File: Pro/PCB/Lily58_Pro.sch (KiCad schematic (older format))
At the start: 83 parts, among them J1 LED, J2 4PIN, J3 OLED, P1 i2c_pin, P2 i2c_pin, SW1 SW_PUSH, SW10 SW_PUSH, SW11 SW_PUSH, SW12 SW_PUSH, SW13 SW_PUSH, SW14 SW_PUSH, SW15 SW_PUSH, SW16 SW_PUSH, SW17 SW_PUSH, SW18 SW_PUSH, SW19 SW_PUSH, SW2 SW_PUSH, SW20 SW_PUSH, SW21 SW_PUSH, SW22 SW_PUSH, SW23 SW_PUSH, SW24 SW_PUSH, SW25 SW_PUSH, SW26 SW_PUSH, SW27 SW_PUSH, SW28 SW_PUSH, SW29 SW_PUSH, SW3 SW_PUSH, SW4 SW_PUSH, SW5 SW_PUSH, SW6 SW_PUSH, SW7 SW_PUSH, SW8 SW_PUSH, SW9 SW_PUSH, U1 ProMicro

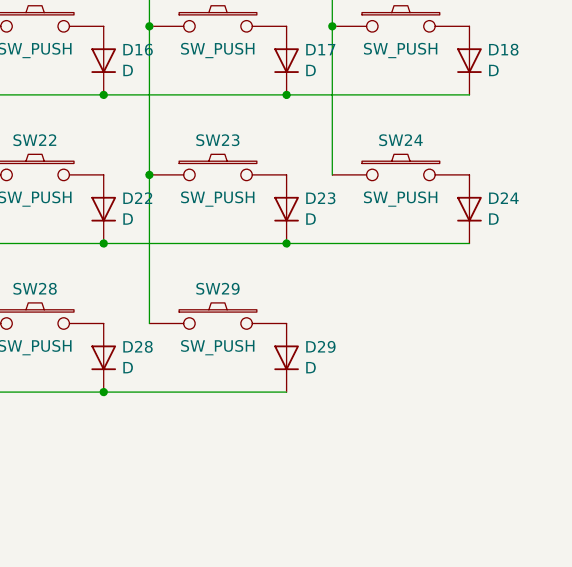
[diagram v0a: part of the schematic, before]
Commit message: Add another switch.
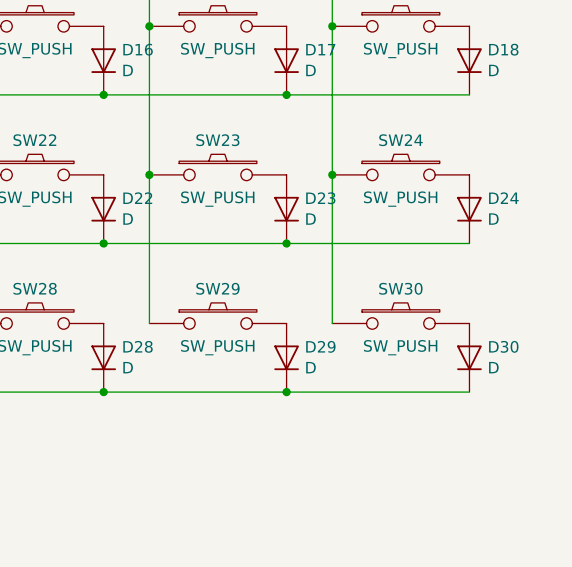
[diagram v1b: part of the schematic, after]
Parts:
- added D30: D, Lily58-footprint:Diode_SOD123, symbol Lily58_Pro-rescue:D-Lily58-cache
- added SW30: SW_PUSH, Lily58-footprint:CherryMX_KailhLowProfile_Hotswap, symbol Lily58_Pro-rescue:SW_PUSH-Lily58-cache
- SW1, SW10, SW11, SW12, SW13, SW14, SW15, SW16, SW17, SW18, SW19, SW2, SW20, SW21, SW22, SW23, SW24, SW25, SW27, SW28, SW29, SW3, SW4, SW5, SW6, SW7, SW8, SW9: footprint Lily58-footprint:CherryMX_KailhLowProfile_Hotswap_edge_fixed -> Lily58-footprint:CherryMX_KailhLowProfile_Hotswap
- SW26: footprint Lily58-footprint:CherryMX_KailhLowProfile_Hotswap_edge_fixed -> Lily58-footprint:CherryMX_KailhLowProfile_Hotswap_1.5
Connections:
- net col0: now also SW30.1
- net row4: now also D30.1 (K)
- new net: D30.2 (A), SW30.2
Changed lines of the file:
@@
 F 0 "SW25" H 5800 5000 50  0000 C CNN
 F 1 "SW_PUSH" H 5800 4750 50  0000 C CNN
-F 2 "Lily58-footprint:CherryMX_KailhLowProfile_Hotswap_edge_fixed" H 5800 4850 50  0001 C CNN
+F 2 "Lily58-footprint:CherryMX_KailhLowProfile_Hotswap" H 5800 4850 50  0001 C CNN
 F 3 "" H 5800 4850 50  0000 C CNN
 	1    5800 4850
@@
 F 0 "SW26" H 6600 5000 50  0000 C CNN
 F 1 "SW_PUSH" H 6600 4750 50  0000 C CNN
-F 2 "Lily58-footprint:CherryMX_KailhLowProfile_Hotswap_edge_fixed" H 6600 4850 50  0001 C CNN
+F 2 "Lily58-footprint:CherryMX_KailhLowProfile_Hotswap_1.5" H 6600 4850 50  0001 C CNN
 F 3 "" H 6600 4850 50  0000 C CNN
 	1    6600 4850
@@
 F 0 "SW1" H 5800 2400 50  0000 C CNN
 F 1 "SW_PUSH" H 5800 2150 50  0000 C CNN
-F 2 "Lily58-footprint:CherryMX_KailhLowProfile_Hotswap_edge_fixed" H 5800 2250 50  0001 C CNN
+F 2 "Lily58-footprint:CherryMX_KailhLowProfile_Hotswap" H 5800 2250 50  0001 C CNN
 F 3 "" H 5800 2250 50  0000 C CNN
 	1    5800 2250
@@
 F 0 "SW2" H 6600 2400 50  0000 C CNN
 F 1 "SW_PUSH" H 6600 2150 50  0000 C CNN
-F 2 "Lily58-footprint:CherryMX_KailhLowProfile_Hotswap_edge_fixed" H 6600 2250 50  0001 C CNN
+F 2 "Lily58-footprint:CherryMX_KailhLowProfile_Hotswap" H 6600 2250 50  0001 C CNN
 F 3 "" H 6600 2250 50  0000 C CNN
 	1    6600 2250
@@
 F 0 "SW3" H 7400 2400 50  0000 C CNN
 F 1 "SW_PUSH" H 7400 2150 50  0000 C CNN
-F 2 "Lily58-footprint:CherryMX_KailhLowProfile_Hotswap_edge_fixed" H 7400 2250 50  0001 C CNN
+F 2 "Lily58-footprint:CherryMX_KailhLowProfile_Hotswap" H 7400 2250 50  0001 C CNN
 F 3 "" H 7400 2250 50  0000 C CNN
 	1    7400 2250
@@
 F 0 "SW4" H 8200 2400 50  0000 C CNN
 F 1 "SW_PUSH" H 8200 2150 50  0000 C CNN
-F 2 "Lily58-footprint:CherryMX_KailhLowProfile_Hotswap_edge_fixed" H 8200 2250 50  0001 C CNN
+F 2 "Lily58-footprint:CherryMX_KailhLowProfile_Hotswap" H 8200 2250 50  0001 C CNN
 F 3 "" H 8200 2250 50  0000 C CNN
 	1    8200 2250
@@
 F 0 "SW5" H 9000 2400 50  0000 C CNN
 F 1 "SW_PUSH" H 9000 2150 50  0000 C CNN
-F 2 "Lily58-footprint:CherryMX_KailhLowProfile_Hotswap_edge_fixed" H 9000 2250 50  0001 C CNN
+F 2 "Lily58-footprint:CherryMX_KailhLowProfile_Hotswap" H 9000 2250 50  0001 C CNN
 F 3 "" H 9000 2250 50  0000 C CNN
 	1    9000 2250
@@
 F 0 "SW6" H 9800 2400 50  0000 C CNN
 F 1 "SW_PUSH" H 9800 2200 50  0000 C CNN
-F 2 "Lily58-footprint:CherryMX_KailhLowProfile_Hotswap_edge_fixed" H 9800 2250 50  0001 C CNN
+F 2 "Lily58-footprint:CherryMX_KailhLowProfile_Hotswap" H 9800 2250 50  0001 C CNN
 F 3 "" H 9800 2250 50  0000 C CNN
 	1    9800 2250
@@
 F 0 "SW8" H 6600 3050 50  0000 C CNN
 F 1 "SW_PUSH" H 6600 2800 50  0000 C CNN
-F 2 "Lily58-footprint:CherryMX_KailhLowProfile_Hotswap_edge_fixed" H 6600 2900 50  0001 C CNN
+F 2 "Lily58-footprint:CherryMX_KailhLowProfile_Hotswap" H 6600 2900 50  0001 C CNN
 F 3 "" H 6600 2900 50  0000 C CNN
 	1    6600 2900
@@
 F 0 "SW9" H 7400 3050 50  0000 C CNN
 F 1 "SW_PUSH" H 7400 2800 50  0000 C CNN
-F 2 "Lily58-footprint:CherryMX_KailhLowProfile_Hotswap_edge_fixed" H 7400 2900 50  0001 C CNN
+F 2 "Lily58-footprint:CherryMX_KailhLowProfile_Hotswap" H 7400 2900 50  0001 C CNN
 F 3 "" H 7400 2900 50  0000 C CNN
 	1    7400 2900
@@
 F 0 "SW10" H 8200 3050 50  0000 C CNN
 F 1 "SW_PUSH" H 8200 2800 50  0000 C CNN
-F 2 "Lily58-footprint:CherryMX_KailhLowProfile_Hotswap_edge_fixed" H 8200 2900 50  0001 C CNN
+F 2 "Lily58-footprint:CherryMX_KailhLowProfile_Hotswap" H 8200 2900 50  0001 C CNN
 F 3 "" H 8200 2900 50  0000 C CNN
 	1    8200 2900
@@
 F 0 "SW11" H 9000 3050 50  0000 C CNN
 F 1 "SW_PUSH" H 9000 2800 50  0000 C CNN
-F 2 "Lily58-footprint:CherryMX_KailhLowProfile_Hotswap_edge_fixed" H 9000 2900 50  0001 C CNN
+F 2 "Lily58-footprint:CherryMX_KailhLowProfile_Hotswap" H 9000 2900 50  0001 C CNN
 F 3 "" H 9000 2900 50  0000 C CNN
 	1    9000 2900
@@
 F 0 "SW12" H 9800 3050 50  0000 C CNN
 F 1 "SW_PUSH" H 9800 2800 50  0000 C CNN
-F 2 "Lily58-footprint:CherryMX_KailhLowProfile_Hotswap_edge_fixed" H 9800 2900 50  0001 C CNN
+F 2 "Lily58-footprint:CherryMX_KailhLowProfile_Hotswap" H 9800 2900 50  0001 C CNN
 F 3 "" H 9800 2900 50  0000 C CNN
 	1    9800 2900
@@
 F 0 "SW7" H 5800 3050 50  0000 C CNN
 F 1 "SW_PUSH" H 5800 2800 50  0000 C CNN
-F 2 "Lily58-footprint:CherryMX_KailhLowProfile_Hotswap_edge_fixed" H 5800 2900 50  0001 C CNN
+F 2 "Lily58-footprint:CherryMX_KailhLowProfile_Hotswap" H 5800 2900 50  0001 C CNN
 F 3 "" H 5800 2900 50  0000 C CNN
 	1    5800 2900
@@
 F 0 "SW13" H 5800 3700 50  0000 C CNN
 F 1 "SW_PUSH" H 5800 3450 50  0000 C CNN
-F 2 "Lily58-footprint:CherryMX_KailhLowProfile_Hotswap_edge_fixed" H 5800 3550 50  0001 C CNN
+F 2 "Lily58-footprint:CherryMX_KailhLowProfile_Hotswap" H 5800 3550 50  0001 C CNN
 F 3 "" H 5800 3550 50  0000 C CNN
 	1    5800 3550
@@
 F 0 "SW14" H 6600 3700 50  0000 C CNN
 F 1 "SW_PUSH" H 6600 3450 50  0000 C CNN
-F 2 "Lily58-footprint:CherryMX_KailhLowProfile_Hotswap_edge_fixed" H 6600 3550 50  0001 C CNN
+F 2 "Lily58-footprint:CherryMX_KailhLowProfile_Hotswap" H 6600 3550 50  0001 C CNN
 F 3 "" H 6600 3550 50  0000 C CNN
 	1    6600 3550
@@
 F 0 "SW15" H 7400 3700 50  0000 C CNN
 F 1 "SW_PUSH" H 7400 3450 50  0000 C CNN
-F 2 "Lily58-footprint:CherryMX_KailhLowProfile_Hotswap_edge_fixed" H 7400 3550 50  0001 C CNN
+F 2 "Lily58-footprint:CherryMX_KailhLowProfile_Hotswap" H 7400 3550 50  0001 C CNN
 F 3 "" H 7400 3550 50  0000 C CNN
 	1    7400 3550
@@
 F 0 "SW16" H 8200 3700 50  0000 C CNN
 F 1 "SW_PUSH" H 8200 3450 50  0000 C CNN
-F 2 "Lily58-footprint:CherryMX_KailhLowProfile_Hotswap_edge_fixed" H 8200 3550 50  0001 C CNN
+F 2 "Lily58-footprint:CherryMX_KailhLowProfile_Hotswap" H 8200 3550 50  0001 C CNN
 F 3 "" H 8200 3550 50  0000 C CNN
 	1    8200 3550
@@
 F 0 "SW17" H 9000 3700 50  0000 C CNN
 F 1 "SW_PUSH" H 9000 3450 50  0000 C CNN
-F 2 "Lily58-footprint:CherryMX_KailhLowProfile_Hotswap_edge_fixed" H 9000 3550 50  0001 C CNN
+F 2 "Lily58-footprint:CherryMX_KailhLowProfile_Hotswap" H 9000 3550 50  0001 C CNN
 F 3 "" H 9000 3550 50  0000 C CNN
 	1    9000 3550
@@
 F 0 "SW18" H 9800 3700 50  0000 C CNN
 F 1 "SW_PUSH" H 9800 3450 50  0000 C CNN
-F 2 "Lily58-footprint:CherryMX_KailhLowProfile_Hotswap_edge_fixed" H 9800 3550 50  0001 C CNN
+F 2 "Lily58-footprint:CherryMX_KailhLowProfile_Hotswap" H 9800 3550 50  0001 C CNN
 F 3 "" H 9800 3550 50  0000 C CNN
 	1    9800 3550
@@
 F 0 "SW21" H 7400 4350 50  0000 C CNN
 F 1 "SW_PUSH" H 7400 4100 50  0000 C CNN
-F 2 "Lily58-footprint:CherryMX_KailhLowProfile_Hotswap_edge_fixed" H 7400 4200 50  0001 C CNN
+F 2 "Lily58-footprint:CherryMX_KailhLowProfile_Hotswap" H 7400 4200 50  0001 C CNN
 F 3 "" H 7400 4200 50  0000 C CNN
 	1    7400 4200
@@
 F 0 "SW22" H 8200 4350 50  0000 C CNN
 F 1 "SW_PUSH" H 8200 4100 50  0000 C CNN
-F 2 "Lily58-footprint:CherryMX_KailhLowProfile_Hotswap_edge_fixed" H 8200 4200 50  0001 C CNN
+F 2 "Lily58-footprint:CherryMX_KailhLowProfile_Hotswap" H 8200 4200 50  0001 C CNN
 F 3 "" H 8200 4200 50  0000 C CNN
 	1    8200 4200
@@
 F 0 "SW23" H 9000 4350 50  0000 C CNN
 F 1 "SW_PUSH" H 9000 4100 50  0000 C CNN
-F 2 "Lily58-footprint:CherryMX_KailhLowProfile_Hotswap_edge_fixed" H 9000 4200 50  0001 C CNN
+F 2 "Lily58-footprint:CherryMX_KailhLowProfile_Hotswap" H 9000 4200 50  0001 C CNN
 F 3 "" H 9000 4200 50  0000 C CNN
 	1    9000 4200
@@
 F 0 "SW24" H 9800 4350 50  0000 C CNN
 F 1 "SW_PUSH" H 9800 4100 50  0000 C CNN
-F 2 "Lily58-footprint:CherryMX_KailhLowProfile_Hotswap_edge_fixed" H 9800 4200 50  0001 C CNN
+F 2 "Lily58-footprint:CherryMX_KailhLowProfile_Hotswap" H 9800 4200 50  0001 C CNN
 F 3 "" H 9800 4200 50  0000 C CNN
 	1    9800 4200
@@
 F 0 "SW20" H 6600 4350 50  0000 C CNN
 F 1 "SW_PUSH" H 6600 4100 50  0000 C CNN
-F 2 "Lily58-footprint:CherryMX_KailhLowProfile_Hotswap_edge_fixed" H 6600 4200 50  0001 C CNN
+F 2 "Lily58-footprint:CherryMX_KailhLowProfile_Hotswap" H 6600 4200 50  0001 C CNN
 F 3 "" H 6600 4200 50  0000 C CNN
 	1    6600 4200
@@
 F 0 "SW19" H 5800 4350 50  0000 C CNN
 F 1 "SW_PUSH" H 5800 4100 50  0000 C CNN
-F 2 "Lily58-footprint:CherryMX_KailhLowProfile_Hotswap_edge_fixed" H 5800 4200 50  0001 C CNN
+F 2 "Lily58-footprint:CherryMX_KailhLowProfile_Hotswap" H 5800 4200 50  0001 C CNN
 F 3 "" H 5800 4200 50  0000 C CNN
 	1    5800 4200
@@
 F 0 "SW27" H 7400 5000 50  0000 C CNN
 F 1 "SW_PUSH" H 7400 4750 50  0000 C CNN
-F 2 "Lily58-footprint:CherryMX_KailhLowProfile_Hotswap_edge_fixed" H 7400 4850 50  0001 C CNN
+F 2 "Lily58-footprint:CherryMX_KailhLowProfile_Hotswap" H 7400 4850 50  0001 C CNN
 F 3 "" H 7400 4850 50  0000 C CNN
 	1    7400 4850
@@
 F 0 "SW28" H 8200 5000 50  0000 C CNN
 F 1 "SW_PUSH" H 8200 4750 50  0000 C CNN
-F 2 "Lily58-footprint:CherryMX_KailhLowProfile_Hotswap_edge_fixed" H 8200 4850 50  0001 C CNN
+F 2 "Lily58-footprint:CherryMX_KailhLowProfile_Hotswap" H 8200 4850 50  0001 C CNN
 F 3 "" H 8200 4850 50  0000 C CNN
 	1    8200 4850
@@
 F 0 "SW29" H 9000 5000 50  0000 C CNN
 F 1 "SW_PUSH" H 9000 4750 50  0000 C CNN
-F 2 "Lily58-footprint:CherryMX_KailhLowProfile_Hotswap_edge_fixed" H 9000 4850 50  0001 C CNN
+F 2 "Lily58-footprint:CherryMX_KailhLowProfile_Hotswap" H 9000 4850 50  0001 C CNN
 F 3 "" H 9000 4850 50  0000 C CNN
 	1    9000 4850
@@
 	3850 2400 4150 2400
 Connection ~ 3550 4550
+$Comp
+L Lily58_Pro-rescue:SW_PUSH-Lily58-cache SW30
+U 1 1 5D954F78
+P 9800 4850
+F 0 "SW30" H 9800 5000 50  0000 C CNN
+F 1 "SW_PUSH" H 9800 4750 50  0000 C CNN
+F 2 "Lily58-footprint:CherryMX_KailhLowProfile_Hotswap" H 9800 4850 50  0001 C CNN
+F 3 "" H 9800 4850 50  0000 C CNN
+	1    9800 4850
+	1    0    0    -1
+$EndComp
+$Comp
+L Lily58_Pro-rescue:D-Lily58-cache D30
+U 1 1 5D956FE1
+P 10100 5000
+F 0 "D30" V 10146 4921 50  0000 R CNN
+F 1 "D" V 10055 4921 50  0000 R CNN
+F 2 "Lily58-footprint:Diode_SOD123" H 10100 5000 50  0001 C CNN
+F 3 "" H 10100 5000 50  0001 C CNN
+	1    10100 5000
+	0    -1   -1   0
+$EndComp
+Wire Wire Line
+	9500 4200 9500 4850
+Connection ~ 9500 4200
+Wire Wire Line
+	9300 5150 10100 5150
+Connection ~ 9300 5150
 $EndSCHEMATC
